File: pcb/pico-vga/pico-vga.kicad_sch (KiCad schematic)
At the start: 42 parts, among them J1 DB15_Female_HighDensity, J2 Micro_SD_Card_Det, J3 USB_A, J4 USB_A, J5 Conn_01x04_Male, J6 AudioJack3, J7 Conn_01x02_Male, J8 USB_A, J9 USB_A, Q1 DMP3099L-7, SW1 SW_Push, U1 Raspberry_Pi_Pico

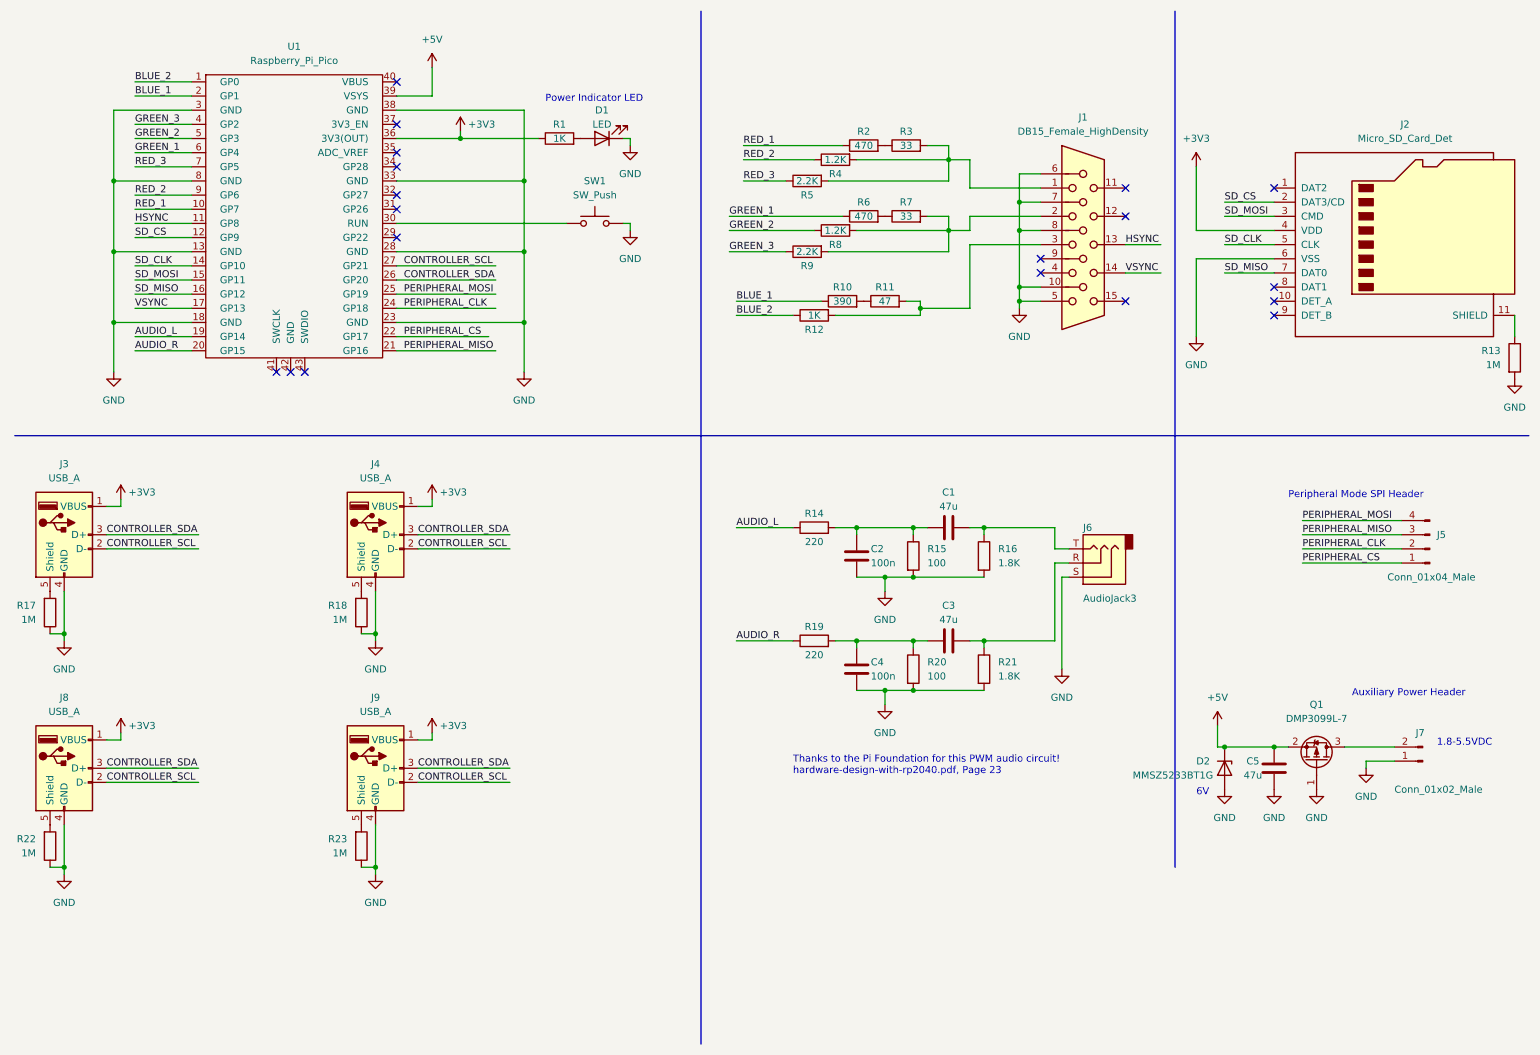
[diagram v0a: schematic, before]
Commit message: Forgot I2C pullup resistors, updated Sch, PCB, and BOM
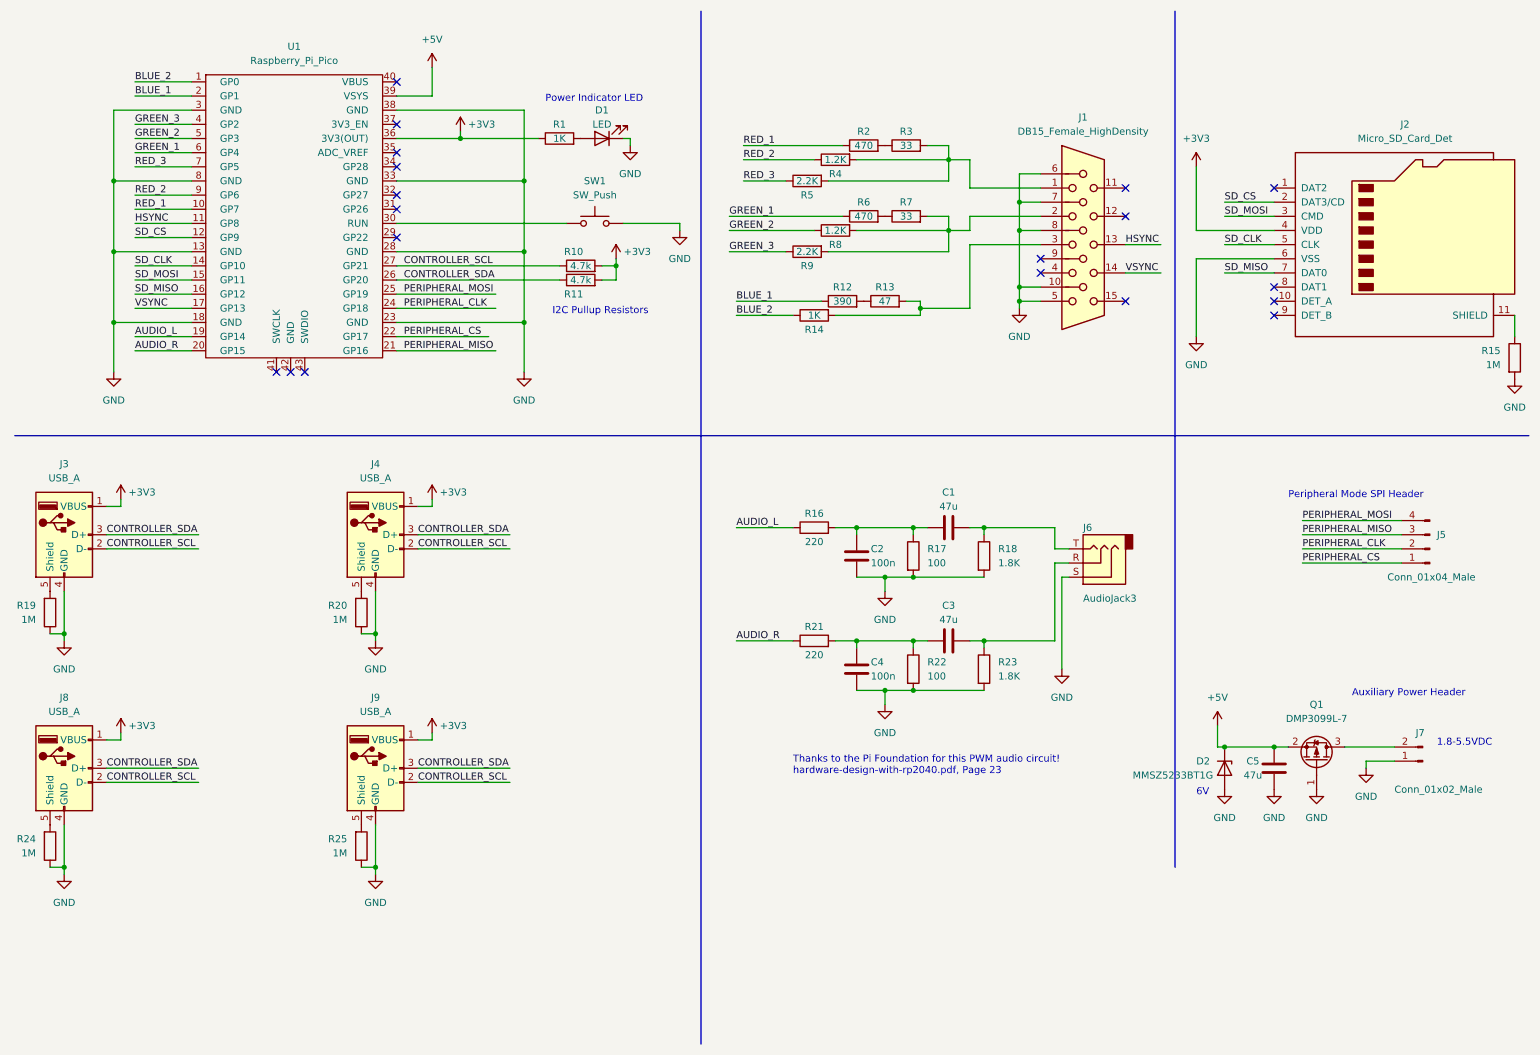
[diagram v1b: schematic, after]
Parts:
- added R10, R11: 4.7k, Resistor_SMD:R_0805_2012Metric_Pad1.20x1.40mm_HandSolder, symbol Device:R
- J2: Part Number (none) -> MEM2061-01-188-00-A
- J6: Part Number SJ1-3533NG -> STX-3000
- renumbered R10 to R12, R11 to R13, R12 to R14, R13 to R15, R14 to R16, R15 to R17, R16 to R18, R17 to R19, R18 to R20, R19 to R21, R20 to R22, R21 to R23, R22 to R24, R23 to R25
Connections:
- net +3V3: now also R10.2, R11.2
- net CONTROLLER_SCL: now also R10.1
- net CONTROLLER_SDA: now also R11.1
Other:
- note added: "I2C Pullup Resistors"

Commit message: Revert "Forgot I2C pullup resistors, updated Sch, PCB, and BOM"
Don't need the pullups, you can do it internally in software. No point adding them and making the BOM longer.

This reverts commit bd8d0dffae4885964e3fb42256447820ac871936.
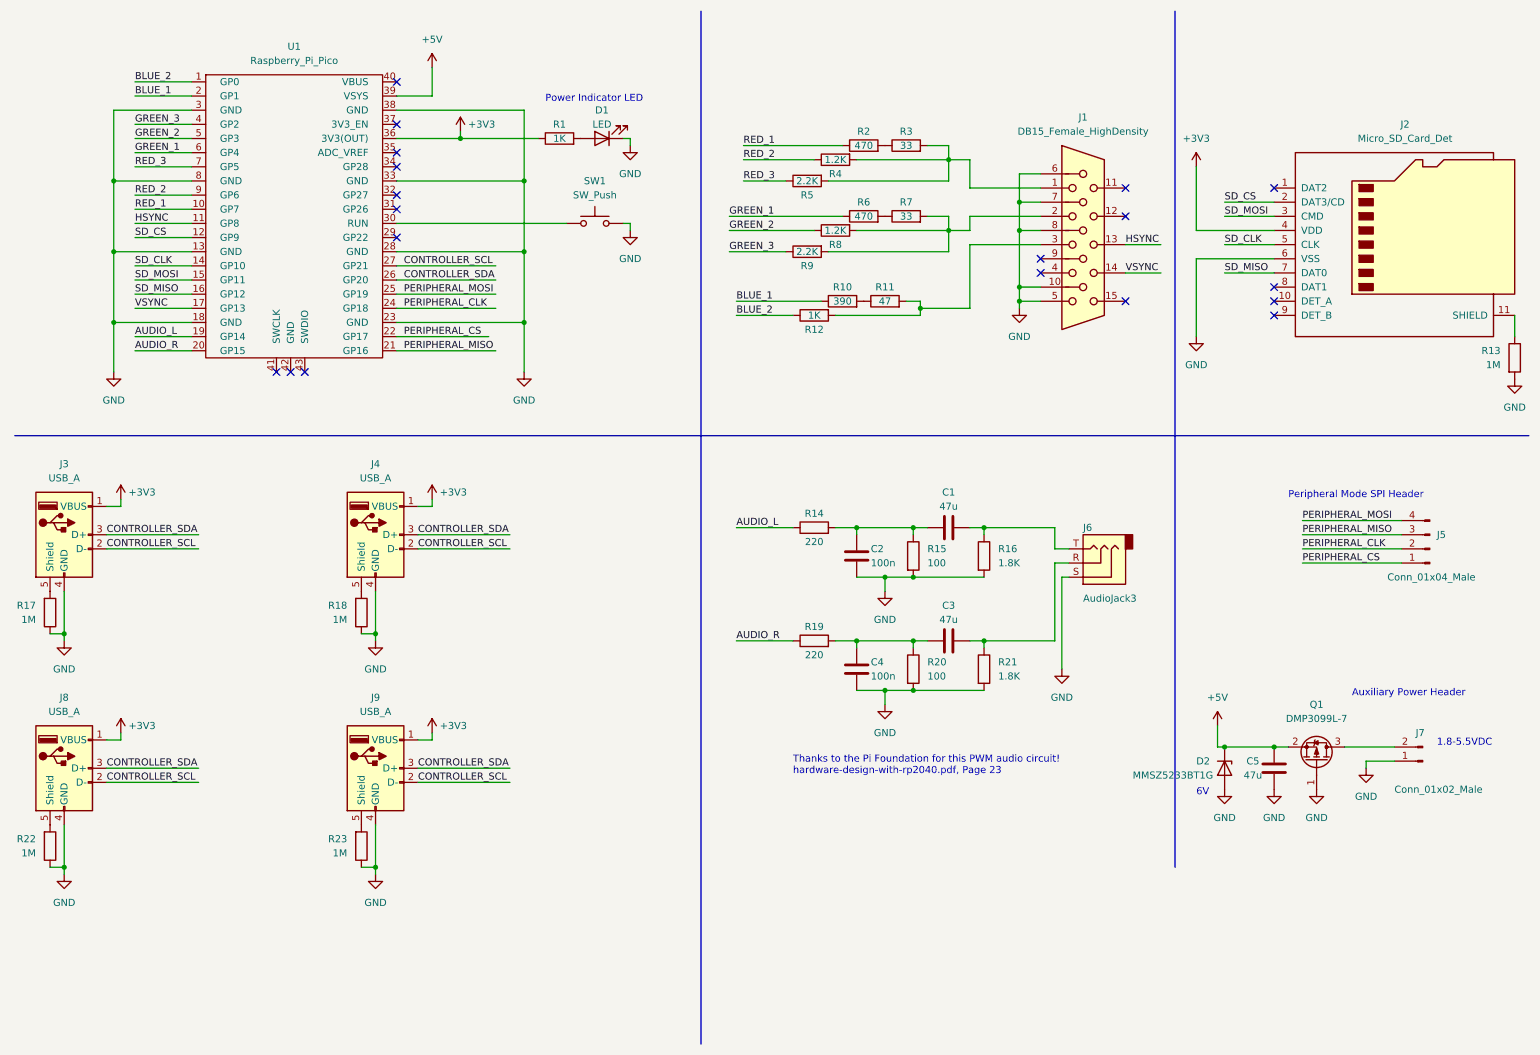
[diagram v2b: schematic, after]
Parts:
- removed R10, R11: 4.7k, Resistor_SMD:R_0805_2012Metric_Pad1.20x1.40mm_HandSolder, symbol Device:R
- J2: Part Number MEM2061-01-188-00-A -> (none)
- J6: Part Number STX-3000 -> SJ1-3533NG
- renumbered R12 to R10, R13 to R11, R14 to R12, R15 to R13, R16 to R14, R17 to R15, R18 to R16, R19 to R17, R20 to R18, R21 to R19, R22 to R20, R23 to R21, R24 to R22, R25 to R23
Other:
- note removed: "I2C Pullup Resistors"
